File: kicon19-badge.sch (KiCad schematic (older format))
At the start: 60 parts, among them J1 LogicProbes, J2 Ports, J6 Conn_ARM_JTAG_SWD_20, J7 USB_B_Micro, SW1 BTN1, SW2 BTN2, SW3 BTN3, SW4 BTN4, SW5 Reset, SW6 Erase, U1 74LCX244MTC, U2 AP3429A, U3 ATSAM4SD16BA-MU, U4 OLED_SSD1306, Y1 12M

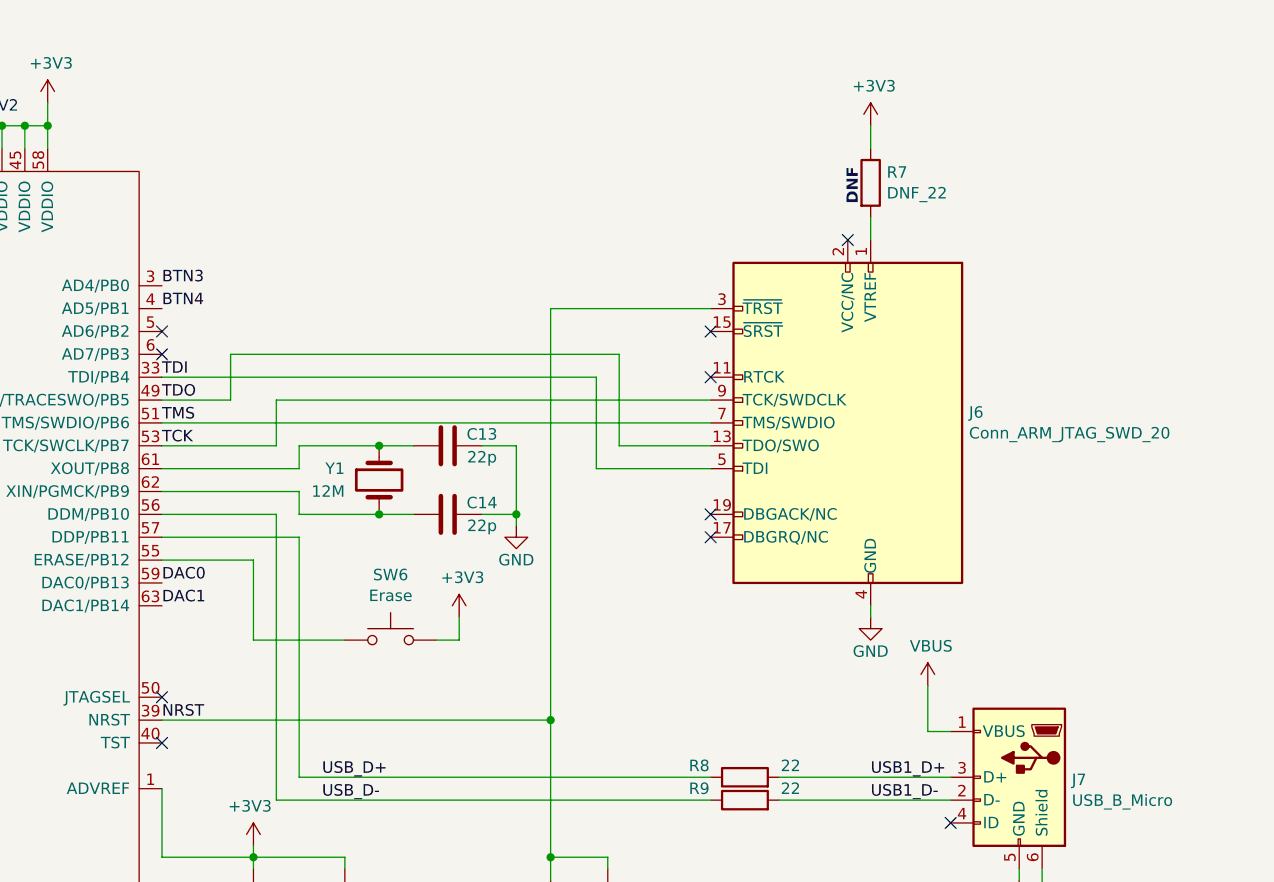
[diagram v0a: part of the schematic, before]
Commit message: WIP
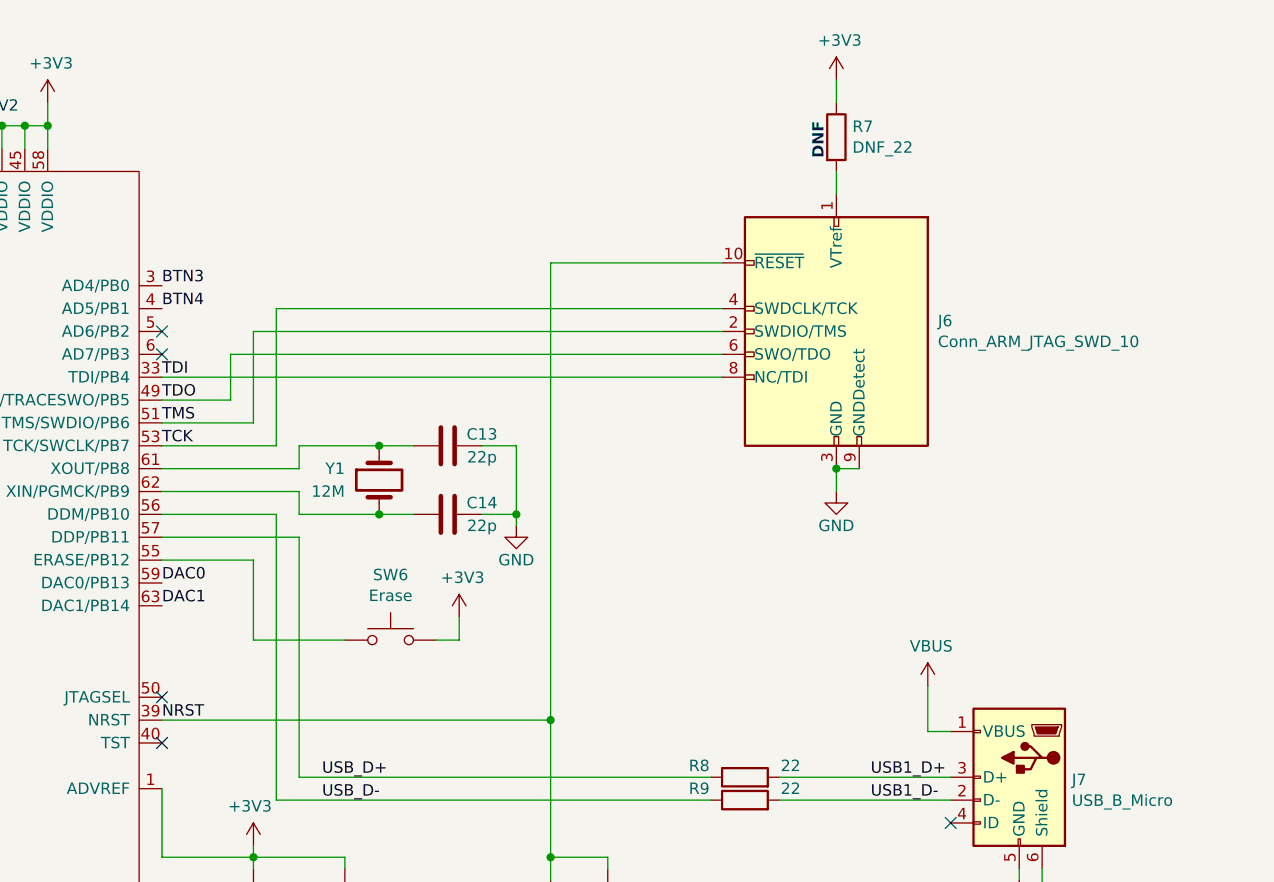
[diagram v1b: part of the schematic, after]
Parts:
- removed J6: Conn_ARM_JTAG_SWD_20, Connector_IDC:IDC-Header_2x10_P2.54mm_Vertical, symbol Connector:Conn_ARM_JTAG_SWD_20
- added J6: Conn_ARM_JTAG_SWD_10, Connector_PinHeader_1.27mm:PinHeader_2x05_P1.27mm_Horizontal, symbol Connector:Conn_ARM_JTAG_SWD_10
- J2: footprint Connector_PinHeader_2.54mm:PinHeader_2x07_P2.54mm_Vertical -> Connector_PinHeader_2.54mm:PinHeader_2x07_P2.54mm_Horizontal
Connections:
- net GND: now also J6.3 (GND), J6.5 (GND), J6.9 (GNDDetect)
- net NRST: now also J6.10 (~RESET~)
- net TCK: now also J6.4 (SWDCLK/TCK)
- net TDI: now also J6.8 (NC/TDI)
- net TDO: now also J6.6 (SWO/TDO)
- net TMS: now also J6.2 (SWDIO/TMS)
- net at R7.2: now also J6.1 (VTref)
- no-connect marks 19 -> 14
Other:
- moved on the sheet: R7
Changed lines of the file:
@@
 $EndDescr
-$Comp
-L Connector:Conn_ARM_JTAG_SWD_20 J6
-U 1 1 5C05E87D
-P 9450 2300
-F 0 "J6" H 8920 2346 50  0000 R CNN
-F 1 "Conn_ARM_JTAG_SWD_20" H 8920 2255 50  0000 R CNN
-F 2 "Connector_IDC:IDC-Header_2x10_P2.54mm_Vertical" H 9900 1250 50  0001 L TNN
-F 3 "http://infocenter.arm.com/help/topic/com.arm.doc.dui0499b/DUI0499B_system_design_reference.pdf" V 9100 1050 50  0001 C CNN
-F 4 "Digi-Key" H 3150 -300 50  0001 C CNN "Distrib1"
-F 5 "ED10524-ND" H 3150 -300 50  0001 C CNN "Distrib1Part"
-F 6 "0.33281" H 3150 -300 50  0001 C CNN "Distrib1Price"
-	1    9450 2300
-	-1   0    0    -1
-$EndComp
 $Comp
 L Device:C C6
@@
 L power:+3V3 #PWR?
 U 1 1 5C0B19FA
-P 9550 1000
+P 9400 800
 AR Path="/5CCA506B/5C0B19FA" Ref="#PWR?"  Part="1"
 AR Path="/5C0B19FA" Ref="#PWR033"  Part="1"
-F 0 "#PWR033" H 9550 850 50  0001 C CNN
-F 1 "+3V3" H 9565 1173 50  0000 C CNN
-F 2 "" H 9550 1000 50  0001 C CNN
-F 3 "" H 9550 1000 50  0001 C CNN
-	1    9550 1000
-	1    0    0    -1
-$EndComp
-NoConn ~ 9450 1500
-NoConn ~ 8850 2700
-NoConn ~ 8850 2800
-$Comp
-L power:GND #PWR034
-U 1 1 5C0EA73C
-P 9550 3150
-F 0 "#PWR034" H 9550 2900 50  0001 C CNN
-F 1 "GND" H 9550 3000 50  0000 C CNN
-F 2 "" H 9550 3150 50  0001 C CNN
-F 3 "" H 9550 3150 50  0001 C CNN
-	1    9550 3150
+F 0 "#PWR033" H 9400 650 50  0001 C CNN
+F 1 "+3V3" H 9415 973 50  0000 C CNN
+F 2 "" H 9400 800 50  0001 C CNN
+F 3 "" H 9400 800 50  0001 C CNN
+	1    9400 800
 	1    0    0    -1
 $EndComp
@@
 	6450 2400 6950 2400
 Wire Wire Line
-	6950 2400 6950 2200
-Wire Wire Line
-	6950 2200 8850 2200
+	6950 2400 6950 1800
 Wire Wire Line
 	6450 2700 6950 2700
@@
 Wire Wire Line
 	7050 3850 8850 3850
-Wire Wire Line
-	8850 1800 8150 1800
-Wire Wire Line
-	8150 1800 8150 3600
 NoConn ~ 6450 3700
 Wire Wire Line
-	9550 3150 9550 3100
-NoConn ~ 8850 1900
-NoConn ~ 8850 2100
-Wire Wire Line
-	6450 2300 8850 2300
-Wire Wire Line
-	6450 2100 8350 2100
-Wire Wire Line
-	8350 2100 8350 2500
-Wire Wire Line
-	8350 2500 8850 2500
-Wire Wire Line
 	6450 2200 6750 2200
-Wire Wire Line
-	8450 2000 8450 2400
-Wire Wire Line
-	8450 2400 8850 2400
 Wire Wire Line
 	3800 4400 4450 4400
@@
 	3800 4000 3800 3500
 Wire Wire Line
-	6750 2000 8450 2000
+	6750 2000 8900 2000
 Wire Wire Line
 	6750 2200 6750 2000
@@
 F 0 "J2" H 1750 2617 50  0000 C CNN
 F 1 "Ports" H 1750 2526 50  0000 C CNN
-F 2 "Connector_PinHeader_2.54mm:PinHeader_2x07_P2.54mm_Vertical" H 1700 2100 50  0001 C CNN
+F 2 "Connector_PinHeader_2.54mm:PinHeader_2x07_P2.54mm_Horizontal" H 1700 2100 50  0001 C CNN
 F 3 "~" H 1700 2100 50  0001 C CNN
 F 4 "Digi-Key" H 100 0   50  0001 C CNN "Distrib1"
@@
 L Device:R R7
 U 1 1 5C2F2686
-P 9550 1250
-F 0 "R7" H 9620 1296 50  0000 L CNN
-F 1 "DNF_22" H 9620 1205 50  0000 L CNN
-F 2 "Resistor_SMD:R_0603_1608Metric" V 9480 1250 50  0001 C CNN
-F 3 "~" H 9550 1250 50  0001 C CNN
-F 4 "Digi-Key" H 3200 -2700 50  0001 C CNN "Distrib1"
-F 5 "CR0603-JW-220ELFCT-ND" H 3200 -2700 50  0001 C CNN "Distrib1Part"
-F 6 "0.0064" H 3200 -2700 50  0001 C CNN "Distrib1Price"
-F 7 "Mouser" H 3200 -2700 50  0001 C CNN "Distrib2"
-F 8 "652-CR0603-JW-220ELF	" H 3200 -2700 50  0001 C CNN "Distrib2Part"
-F 9 "0.006" H 3200 -2700 50  0001 C CNN "Distrib2Price"
-F 10 "No" H 9550 1250 50  0001 C CNN "Mounted"
-	1    9550 1250
-	1    0    0    -1
-$EndComp
-Wire Wire Line
-	9550 1400 9550 1500
-Wire Wire Line
-	9550 1000 9550 1100
+P 9400 1050
+F 0 "R7" H 9470 1096 50  0000 L CNN
+F 1 "DNF_22" H 9470 1005 50  0000 L CNN
+F 2 "Resistor_SMD:R_0603_1608Metric" V 9330 1050 50  0001 C CNN
+F 3 "~" H 9400 1050 50  0001 C CNN
+F 4 "Digi-Key" H 3050 -2900 50  0001 C CNN "Distrib1"
+F 5 "CR0603-JW-220ELFCT-ND" H 3050 -2900 50  0001 C CNN "Distrib1Part"
+F 6 "0.0064" H 3050 -2900 50  0001 C CNN "Distrib1Price"
+F 7 "Mouser" H 3050 -2900 50  0001 C CNN "Distrib2"
+F 8 "652-CR0603-JW-220ELF	" H 3050 -2900 50  0001 C CNN "Distrib2Part"
+F 9 "0.006" H 3050 -2900 50  0001 C CNN "Distrib2Price"
+F 10 "No" H 9400 1050 50  0001 C CNN "Mounted"
+	1    9400 1050
+	1    0    0    -1
+$EndComp
+Wire Wire Line
+	9400 1200 9400 1300
+Wire Wire Line
+	9400 800  9400 900
 NoConn ~ 6450 3500
 Connection ~ 8150 4200
@@
 Wire Wire Line
 	1000 5000 900  5000
-Text Notes 9500 1350 1    50   ~ 10
+Text Notes 9350 1150 1    50   ~ 10
 DNF
 Wire Wire Line
@@
 	-1   0    0    1
 $EndComp
+Text Notes 7000 7100 0    50   ~ 0
+Copyright Maciej Suminski 2019\nThis documentation describes Open Hardware and is licensed under the CERN OHL v. 1.2.\nYou may redistribute and modify this documentation under the terms of the\nCERN OHL v.1.2. (http://ohwr.org/cernohl). This documentation is distributed\nWITHOUT ANY EXPRESS OR IMPLIED WARRANTY, INCLUDING OF MERCHANTABILITY,\nSATISFACTORY QUALITY AND FITNESS FOR A PARTICULAR PURPOSE.\nPlease see the CERN OHL v.1.2 for applicable conditions.
+$Comp
+L power:GND #PWR034
+U 1 1 5C0EA73C
+P 9400 2600
+F 0 "#PWR034" H 9400 2350 50  0001 C CNN
+F 1 "GND" H 9400 2450 50  0000 C CNN
+F 2 "" H 9400 2600 50  0001 C CNN
+F 3 "" H 9400 2600 50  0001 C CNN
+	1    9400 2600
+	1    0    0    -1
+$EndComp
+Wire Wire Line
+	6950 1800 8900 1800
+$Comp
+L Connector:Conn_ARM_JTAG_SWD_10 J6
+U 1 1 5CC9E578
+P 9400 1900
+F 0 "J6" H 8956 1946 50  0000 R CNN
+F 1 "Conn_ARM_JTAG_SWD_10" H 8956 1855 50  0000 R CNN
+F 2 "Connector_PinHeader_1.27mm:PinHeader_2x05_P1.27mm_Horizontal" H 9400 1900 50  0001 C CNN
+F 3 "http://infocenter.arm.com/help/topic/com.arm.doc.ddi0314h/DDI0314H_coresight_components_trm.pdf" V 9050 650 50  0001 C CNN
+	1    9400 1900
+	-1   0    0    -1
+$EndComp
+Wire Wire Line
+	8900 1600 8150 1600
+Wire Wire Line
+	8150 1600 8150 3600
+Wire Wire Line
+	6450 2100 8900 2100
+Wire Wire Line
+	6450 2300 6850 2300
+Wire Wire Line
+	6850 2300 6850 1900
+Wire Wire Line
+	6850 1900 8900 1900
+Wire Wire Line
+	9400 2600 9400 2500
+Wire Wire Line
+	9400 2500 9500 2500
 Wire Bus Line
 	1500 4000 1500 4700
 Wire Bus Line
 	2200 4000 2200 4700
-Text Notes 7000 7100 0    50   ~ 0
-Copyright Maciej Suminski 2019\nThis documentation describes Open Hardware and is licensed under the CERN OHL v. 1.2.\nYou may redistribute and modify this documentation under the terms of the\nCERN OHL v.1.2. (http://ohwr.org/cernohl). This documentation is distributed\nWITHOUT ANY EXPRESS OR IMPLIED WARRANTY, INCLUDING OF MERCHANTABILITY,\nSATISFACTORY QUALITY AND FITNESS FOR A PARTICULAR PURPOSE.\nPlease see the CERN OHL v.1.2 for applicable conditions.
+Connection ~ 9400 2500
 $EndSCHEMATC
